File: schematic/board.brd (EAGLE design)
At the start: 80 x 80 mm, 22 parts, among them U1 STM32F103C8T6

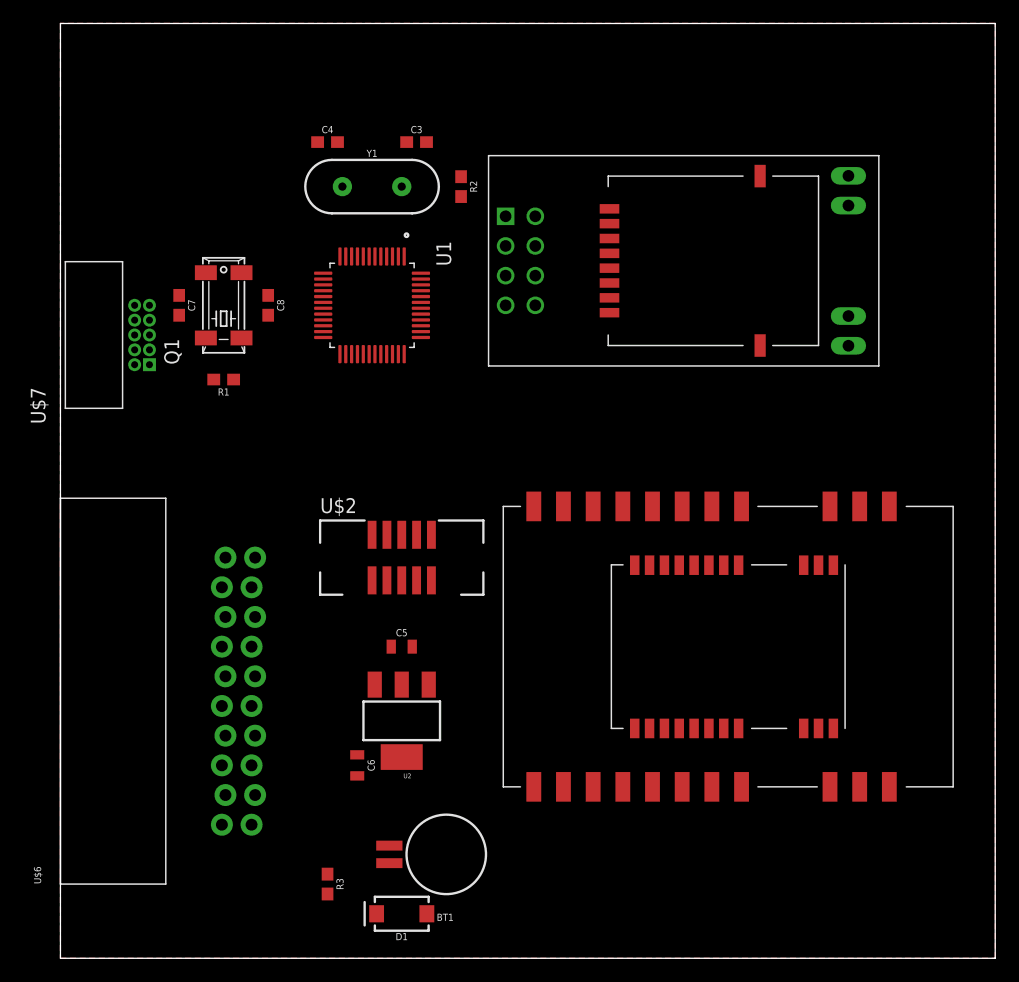
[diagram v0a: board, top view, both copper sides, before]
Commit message: Прикидки размеров платы
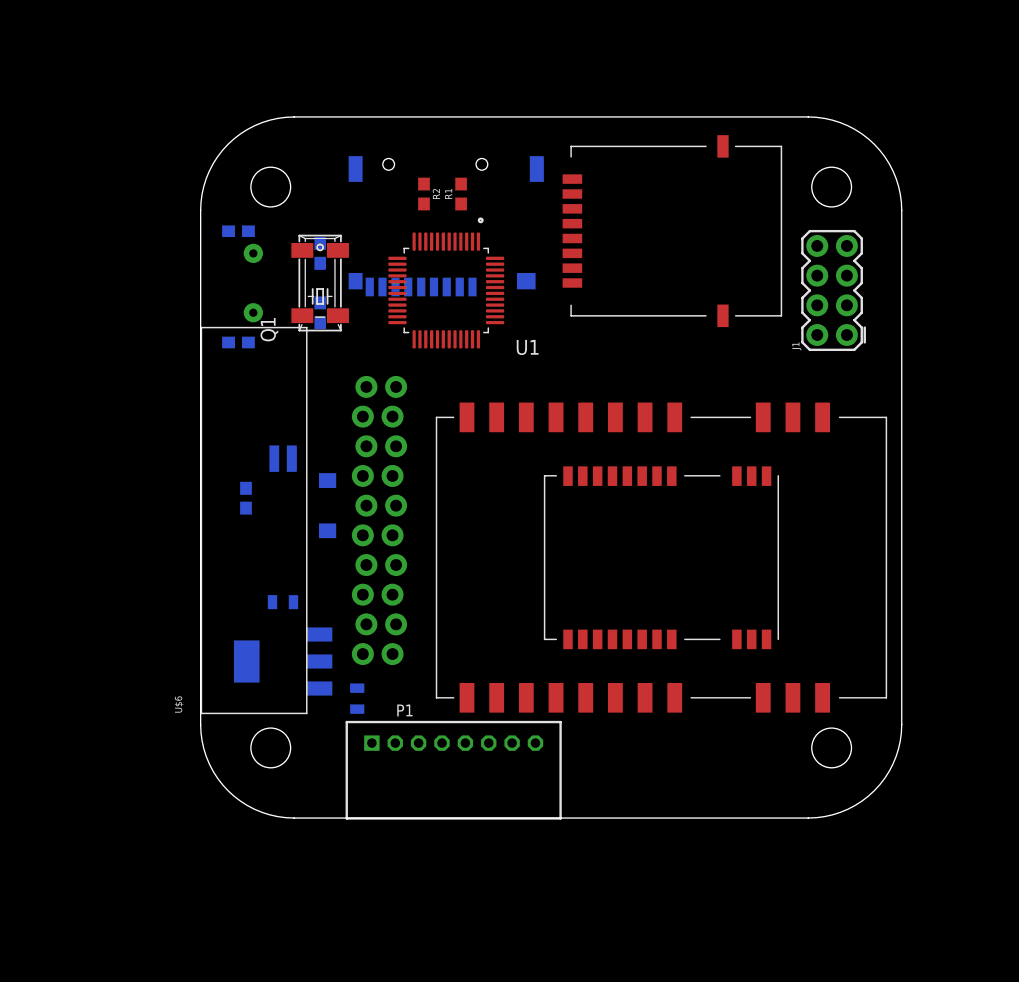
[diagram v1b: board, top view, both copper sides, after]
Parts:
- removed U$5: E01-ML01DP5, ebyte-radio:E01-ML01DP5/E01-2G4M27D
- removed U$7: CST2-JTAG2X5-1.27MM-R, IDC:2X5-1.27MM-R
- added J1: (no value), SparkFun-Connectors:2X4
- added P1: S8B-PH-K, con-jst-ph:S8B-PH-K
- U$2: value CST2-JTAG -> TFP09-2-12B; device IDC:2X5-1.27MM-SMT -> sdcard:TFP09-2-12B
- moved BT1 41.2 mm to (19.1, 47.6), flipped to the bottom, turned to 270 degrees
- moved D1 35.5 mm to (22.9, 38.7), flipped to the bottom, turned to 90 degrees
- moved U$2 33.9 mm to (33.0, 67.9), flipped to the bottom, turned to 180 degrees
- moved R3 33.8 mm to (15.9, 39.4), flipped to the bottom
- moved R1 25.8 mm to (34.3, 65.4), turned to 90 degrees
- moved U$6 18.9 mm to (27.3, 37.5)
- moved C4 18.8 mm to (15.2, 52.7), flipped to the bottom
- moved C3 17.0 mm to (15.2, 62.2), flipped to the bottom
- moved C6 15.3 mm to (19.1, 30.5), flipped to the bottom, turned to 180 degrees
- moved Y1 13.1 mm to (16.5, 57.8), flipped to the bottom, turned to 90 degrees
- moved C7 12.9 mm to (22.2, 60.3), flipped to the bottom
- moved U2 11.4 mm to (19.1, 25.4), flipped to the bottom, turned to 270 degrees
- moved U$1 9.52 mm to (51.4, 34.3)
- moved U$3 9.52 mm to (51.4, 34.3)
- moved Q1 8.47 mm to (22.2, 57.8)
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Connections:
- net +3V3: no longer U$2.1
- net +5V: no longer U$2.3
- net GND: no longer U$2.9, U$5.1
- net JTCK: no longer U$2.4
- net JTDI: no longer U$2.8
- net JTDO: no longer U$2.6
- net JTMS: no longer U$2.2
- net NRST: no longer U$2.10
- net VCC: no longer U$5.2
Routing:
- removed copper zone on layer 1, net GND
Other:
- board size 80 x 80 mm -> 60 x 60 mm
